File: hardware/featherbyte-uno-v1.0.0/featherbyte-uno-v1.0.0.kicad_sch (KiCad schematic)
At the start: 60 parts, among them J1 Conn_01x08, J10 Conn_01x09, J2 Conn_01x10, J3 Conn_01x06, J5 USB_C_Receptacle_16P, J6 SWD Connector, J7 Terminal Block, J8 USB_C_Receptacle_16P, J9 BOOT1, SW1 Reset, SW2 BOOT0, SW3 SW_DIP_x04, U1 CH32V203CxT6, U2 TJA1050, U4 AMS1117-3.3, U5 USBLC6-2P6, U6 USBLC6-2P6, Y1 8M, Y3 32.768K

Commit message: version info addition and adc pin correction done
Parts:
- JP1, JP2, JP3: now in the parts list

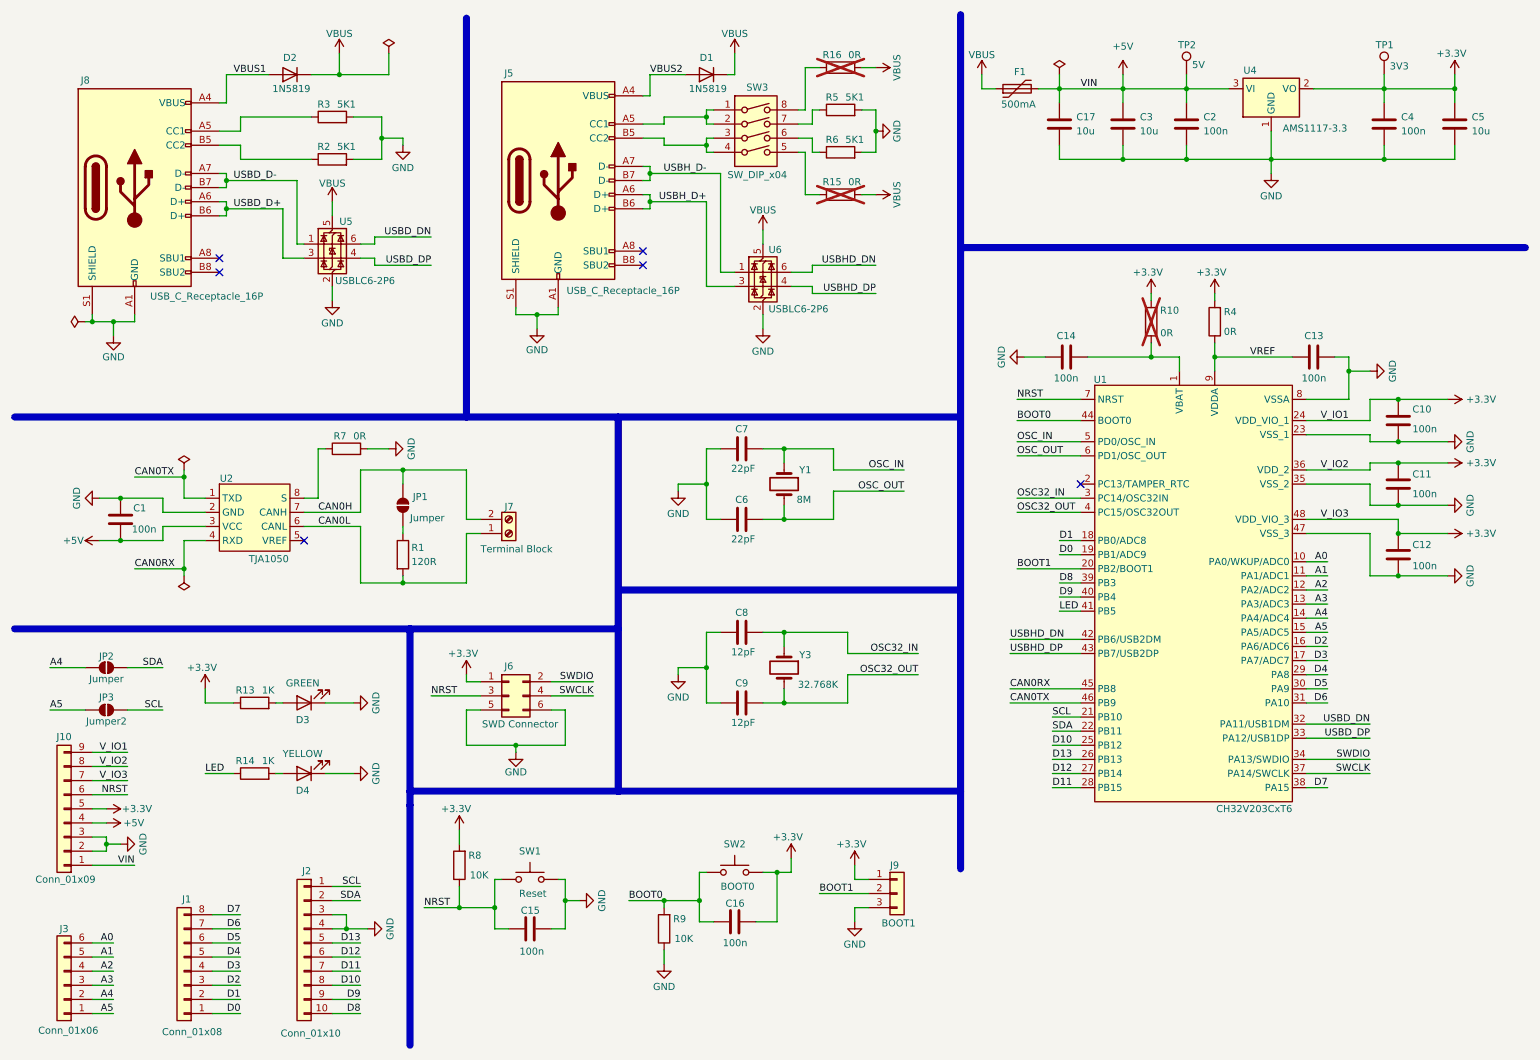
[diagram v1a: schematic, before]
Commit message: schematics updated for visual reasons
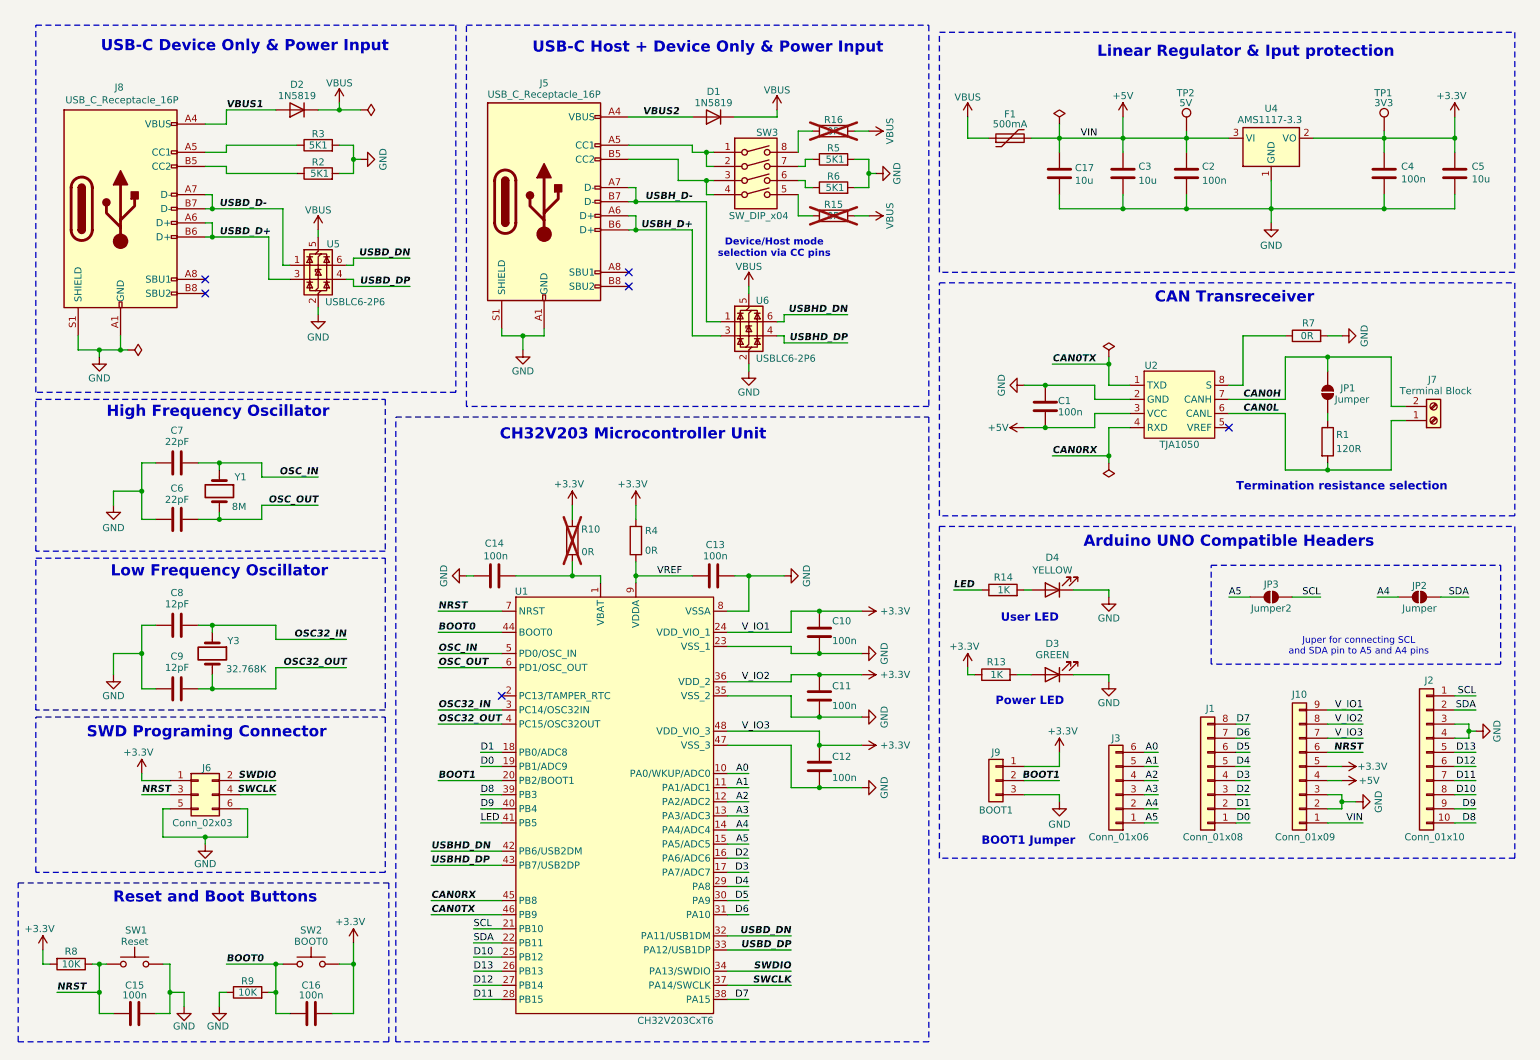
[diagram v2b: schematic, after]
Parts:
- J6: value SWD Connector -> Conn_02x03
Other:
- note added: "Arduino UNO Compatible Headers"
- note added: "BOOT1 Jumper"
- note added: "CAN Transreceiver"
- note added: "CH32V203 Microcontroller Unit"
- note added: "Device/Host mode selection via CC pins"
- note added: "High Frequency Oscillator"
- note added: "Juper for connecting SCL and SDA pin to A5 and A4 pins"
- note added: "Linear Regulator & Iput protection"
- note added: "Low Frequency Oscillator"
- note added: "Power LED"
- note added: "Reset and Boot Buttons"
- note added: "SWD Programing Connector"
- note added: "Termination resistance selection"
- note added: "USB-C Device Only & Power Input"
- note added: "USB-C Host + Device Only & Power Input"
- note added: "User LED"
- title: featherbyte-uno Root -> featherbyte-uno
- moved on the sheet: C1, C10, C11, C12, C13, C14, C15, C16, C17, C2, C3, C4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
